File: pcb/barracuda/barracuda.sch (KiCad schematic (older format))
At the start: 81 parts, among them J1 USB_B_Micro, SW1 SW_PUSH, SW10 SW_PUSH, SW11 SW_PUSH, SW12 SW_PUSH, SW13 SW_PUSH, SW14 SW_PUSH, SW15 SW_PUSH, SW16 SW_PUSH, SW17 SW_PUSH, SW18 SW_PUSH, SW19 SW_PUSH, SW2 SW_PUSH, SW20 SW_PUSH, SW21 SW_PUSH, SW22 SW_PUSH, SW23 SW_PUSH, SW24 SW_PUSH, SW25 SW_PUSH, SW26 SW_PUSH, SW27 SW_PUSH, SW28 SW_PUSH, SW29 SW_PUSH, SW3 SW_PUSH, SW30 SW_PUSH, SW31 SW_PUSH, SW32 SW_PUSH, SW33 SW_PUSH, SW4 SW_PUSH, SW5 SW_PUSH, SW6 SW_PUSH, SW7 SW_PUSH, SW8 SW_PUSH, SW9 SW_PUSH, U1 ATmega32U2-AU, Y1 Crystal_GND24_Small

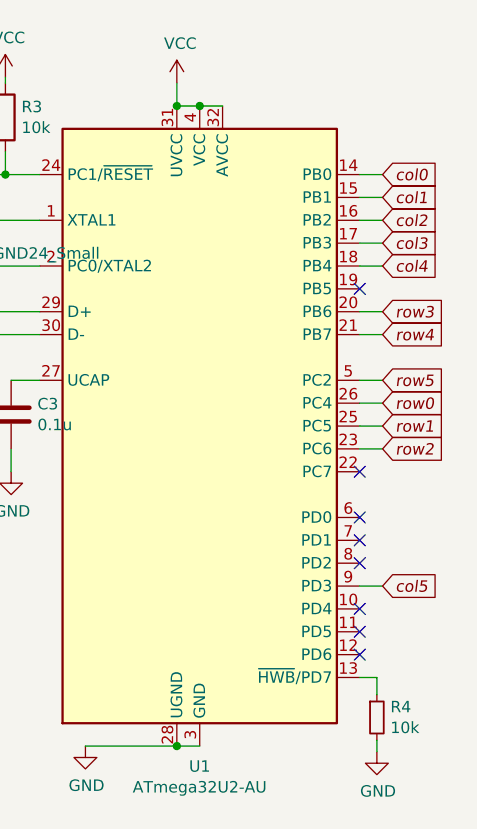
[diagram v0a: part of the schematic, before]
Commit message: save
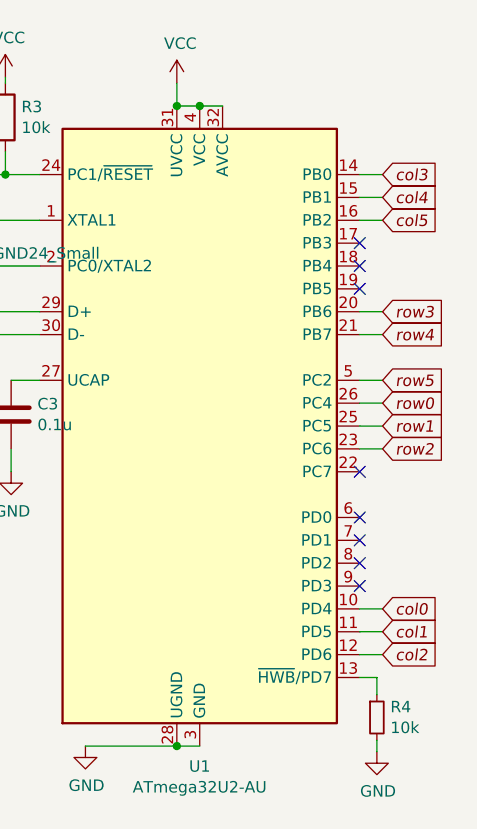
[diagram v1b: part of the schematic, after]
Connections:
- net col0: now also U1.10 (PD4); no longer U1.14 (PB0)
- net col1: now also U1.11 (PD5); no longer U1.15 (PB1)
- net col2: now also U1.12 (PD6); no longer U1.16 (PB2)
- net col3: now also U1.14 (PB0); no longer U1.17 (PB3)
- net col4: now also U1.15 (PB1); no longer U1.18 (PB4)
- net col5: now also U1.16 (PB2); no longer U1.9 (PD3)
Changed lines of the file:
@@
 Text GLabel 10950 4250 2    50   Input Italic 0
 row5
+Text GLabel 10950 5250 2    50   Input Italic 0
+col0
+Text GLabel 10950 5350 2    50   Input Italic 0
+col1
+Text GLabel 10950 5450 2    50   Input Italic 0
+col2
 Text GLabel 10950 3350 2    50   Input Italic 0
-col0
+col3
 Text GLabel 10950 3450 2    50   Input Italic 0
-col1
+col4
 Text GLabel 10950 3550 2    50   Input Italic 0
-col2
-Text GLabel 10950 3650 2    50   Input Italic 0
-col3
-Text GLabel 10950 3750 2    50   Input Italic 0
-col4
-Text GLabel 10950 5150 2    50   Input Italic 0
 col5
 Connection ~ 3350 1575
@@
 Connection ~ 10150 3050
 Wire Wire Line
-	10850 3350 10950 3350
-Wire Wire Line
-	10850 3450 10950 3450
-Wire Wire Line
-	10850 3550 10950 3550
-Wire Wire Line
-	10850 3650 10950 3650
-Wire Wire Line
-	10850 3750 10950 3750
-Wire Wire Line
 	10850 3950 10950 3950
 Wire Wire Line
@@
 NoConn ~ 10850 4950
 NoConn ~ 10850 5050
-NoConn ~ 10850 5250
-NoConn ~ 10850 5350
-NoConn ~ 10850 5450
 $Comp
 L Connector:USB_B_Micro J1
@@
 Wire Wire Line
 	950  6600 950  6800
-Wire Wire Line
-	10850 5150 10950 5150
 NoConn ~ 10850 3850
 $Comp
@@
 Wire Wire Line
 	10925 5825 10925 5875
+Wire Wire Line
+	10850 3550 10950 3550
+Wire Wire Line
+	10850 3450 10950 3450
+Wire Wire Line
+	10850 3350 10950 3350
+Wire Wire Line
+	10850 5450 10950 5450
+Wire Wire Line
+	10850 5250 10950 5250
+Wire Wire Line
+	10850 5350 10950 5350
+NoConn ~ 10850 3650
+NoConn ~ 10850 3750
+NoConn ~ 10850 5150
 $EndSCHEMATC

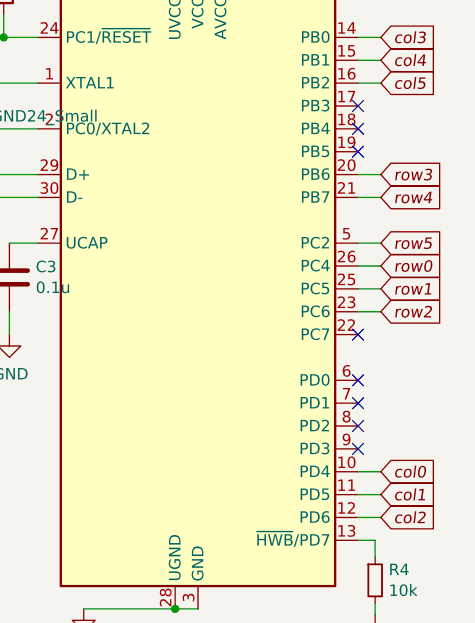
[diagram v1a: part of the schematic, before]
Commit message: Finished routing
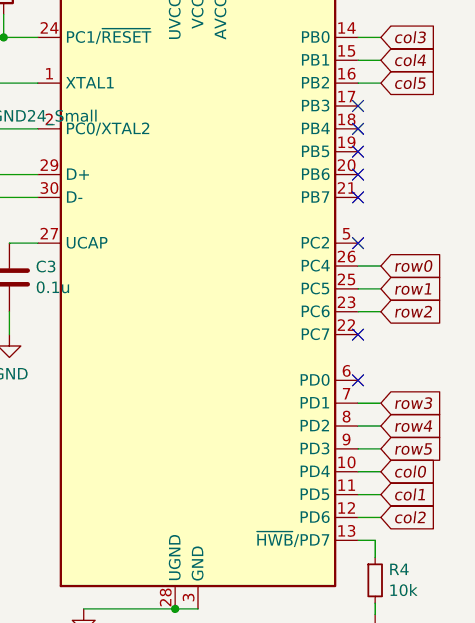
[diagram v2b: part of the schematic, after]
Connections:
- net row3: now also U1.7 (PD1); no longer U1.20 (PB6)
- net row4: now also U1.8 (PD2); no longer U1.21 (PB7)
- net row5: now also U1.9 (PD3); no longer U1.5 (PC2)
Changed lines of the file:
@@
 Text GLabel 10950 4550 2    50   Input Italic 0
 row2
-Text GLabel 10950 3950 2    50   Input Italic 0
+Text GLabel 10950 4950 2    50   Input Italic 0
 row3
-Text GLabel 10950 4050 2    50   Input Italic 0
+Text GLabel 10950 5050 2    50   Input Italic 0
 row4
-Text GLabel 10950 4250 2    50   Input Italic 0
+Text GLabel 10950 5150 2    50   Input Italic 0
 row5
 Text GLabel 10950 5250 2    50   Input Italic 0
@@
 Connection ~ 10150 3050
 Wire Wire Line
-	10850 3950 10950 3950
-Wire Wire Line
-	10850 4050 10950 4050
-Wire Wire Line
-	10850 4250 10950 4250
-Wire Wire Line
 	10850 4350 10950 4350
 Wire Wire Line
@@
 NoConn ~ 10850 4650
 NoConn ~ 10850 4850
-NoConn ~ 10850 4950
-NoConn ~ 10850 5050
 $Comp
 L Connector:USB_B_Micro J1
@@
 NoConn ~ 10850 3650
 NoConn ~ 10850 3750
-NoConn ~ 10850 5150
+Wire Wire Line
+	10850 4950 10950 4950
+Wire Wire Line
+	10850 5050 10950 5050
+Wire Wire Line
+	10850 5150 10950 5150
+NoConn ~ 10850 3950
+NoConn ~ 10850 4050
+NoConn ~ 10850 4250
 $EndSCHEMATC
